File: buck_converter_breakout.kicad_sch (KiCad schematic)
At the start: 36 parts, among them J1 XT-60, J2 Conn_01x02, Q1 NMOS, Q2 PMOS, U1 MIC24066T-E/QNA

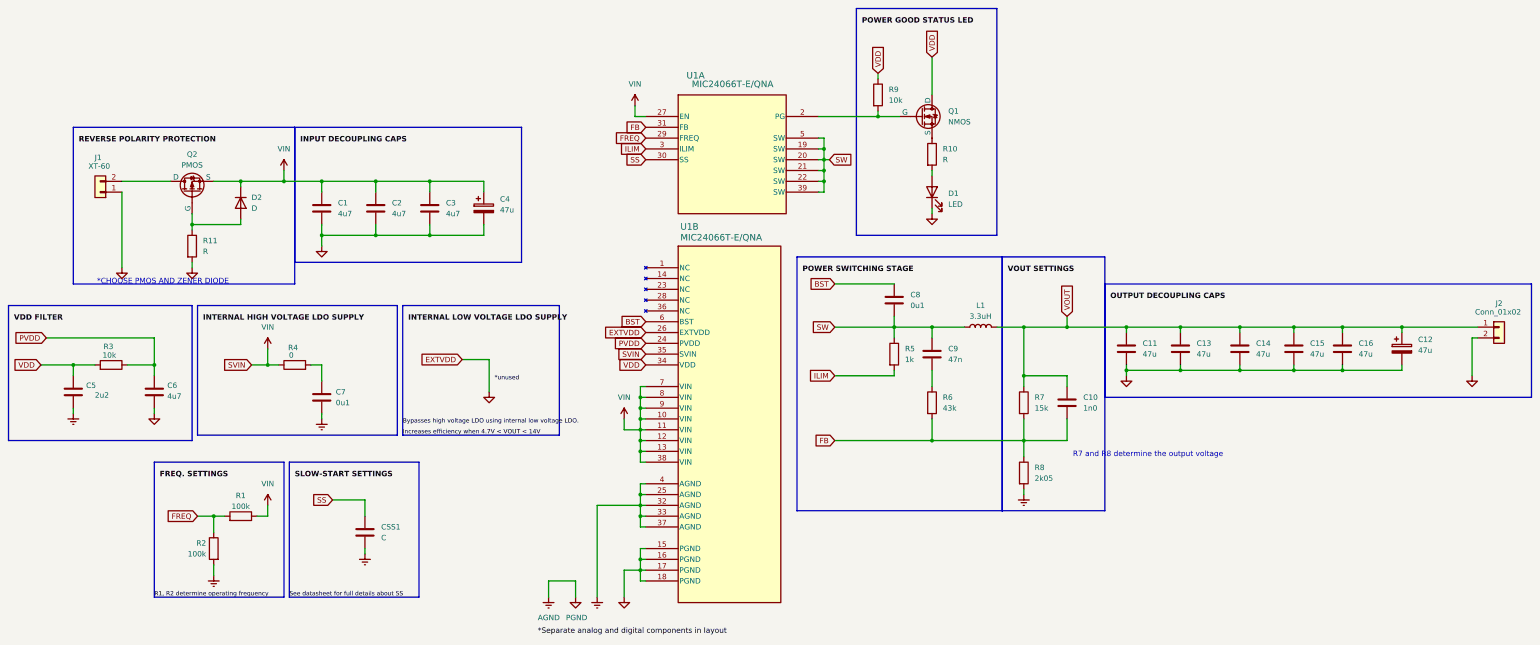
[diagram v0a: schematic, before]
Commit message: completed basic layout
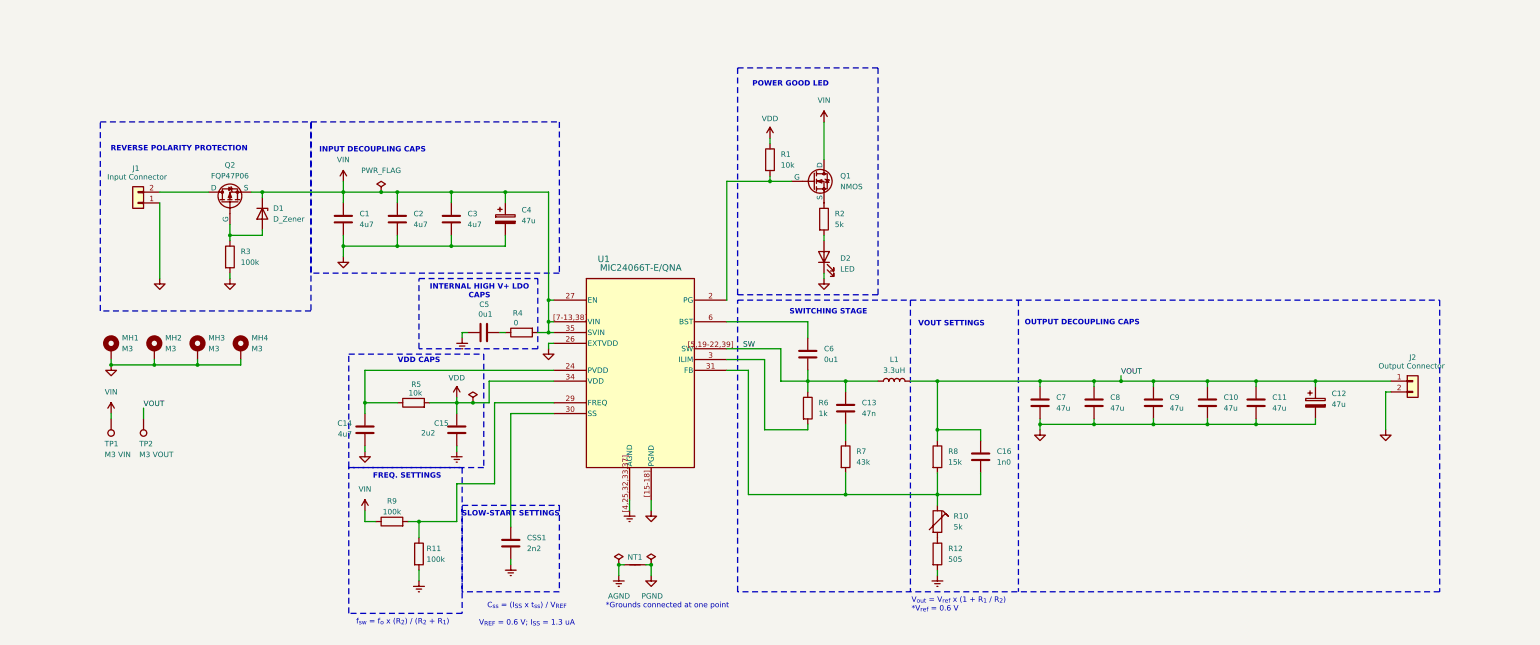
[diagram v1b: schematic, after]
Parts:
- removed D2: D, symbol Device:D
- removed unit 2 of U1
- added D1: D_Zener, Diode_SMD:D_SOD-323, symbol Device:D_Zener
- added MH1, MH2, MH3, MH4: M3, MountingHole:MountingHole_3.2mm_M3_ISO7380_Pad, symbol Mechanical:MountingHole_Pad
- added NT1: NetTie_2, NetTie:NetTie-2_SMD_Pad0.5mm, symbol Device:NetTie_2
- added R10: 5k, Potentiometer_SMD:Potentiometer_Bourns_3314J_Vertical, symbol Device:R_Trim
- added TP1: M3 VIN, TestPoint:TestPoint_Loop_D2.50mm_Drill1.0mm, symbol Connector:TestPoint
- added TP2: M3 VOUT, TestPoint:TestPoint_Loop_D2.50mm_Drill1.0mm, symbol Connector:TestPoint
- C1, C2, C3: footprint (none) -> Capacitor_SMD:C_1210_3225Metric
- C10: renamed from C15; footprint (none) -> Capacitor_SMD:C_1210_3225Metric
- C11: renamed from C16; footprint (none) -> Capacitor_SMD:C_1210_3225Metric
- C12, C4: footprint (none) -> Capacitor_SMD:CP_Elec_6.3x7.7
- C13: renamed from C9; footprint (none) -> Capacitor_SMD:C_0402_1005Metric
- C14: renamed from C6; footprint (none) -> Capacitor_SMD:C_01005_0402Metric
- C15: renamed from C5; footprint (none) -> Capacitor_SMD:C_0201_0603Metric
- C16: renamed from C10; footprint (none) -> Capacitor_SMD:C_0603_1608Metric
- C5: renamed from C7; footprint (none) -> Capacitor_SMD:C_0201_0603Metric
- C6: renamed from C8; footprint (none) -> Capacitor_SMD:C_0402_1005Metric
- C7: renamed from C11; footprint (none) -> Capacitor_SMD:C_1210_3225Metric
- C8: renamed from C13; footprint (none) -> Capacitor_SMD:C_1210_3225Metric
- C9: renamed from C14; footprint (none) -> Capacitor_SMD:C_1210_3225Metric
- CSS1: value C -> 2n2; footprint (none) -> Capacitor_SMD:C_0402_1005Metric
- D2: renamed from D1; footprint (none) -> Capacitor_SMD:C_0805_2012Metric
- J1: value XT-60 -> Input Connector; footprint (none) -> Connector_AMASS:AMASS_XT60-F_1x02_P7.20mm_Vertical
- J2: value Conn_01x02 -> Output Connector; footprint (none) -> Connector_AMASS:AMASS_XT60-F_1x02_P7.20mm_Vertical
- L1: footprint (none) -> Inductor_SMD:XGL6060-332MEC
- Q1: footprint (none) -> Package_TO_SOT_SMD:SOT-23-3
- Q2: value PMOS -> FQP47P06; footprint (none) -> Package_TO_SOT_THT:TO-220-3_Horizontal_TabDown
- R1: renamed from R9; footprint (none) -> Resistor_SMD:R_0603_1608Metric
- R11: renamed from R2; footprint (none) -> Resistor_SMD:R_0603_1608Metric
- R12: renamed from R8; value 2k05 -> 505; footprint (none) -> Resistor_SMD:R_0603_1608Metric
- R2: renamed from R10; value R -> 5k; footprint (none) -> Resistor_SMD:R_0603_1608Metric
- R3: renamed from R11; value R -> 100k; footprint (none) -> Resistor_SMD:R_0603_1608Metric
- R4: footprint (none) -> Resistor_SMD:R_0603_1608Metric
- R5: renamed from R3; footprint (none) -> Resistor_SMD:R_0603_1608Metric
- R6: renamed from R5; footprint (none) -> Resistor_SMD:R_0603_1608Metric
- R7: renamed from R6; footprint (none) -> Resistor_SMD:R_0603_1608Metric
- R8: renamed from R7; footprint (none) -> Resistor_SMD:R_0603_1608Metric
- R9: renamed from R1; footprint (none) -> Resistor_SMD:R_0603_1608Metric
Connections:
- net AGND: now also C5.1, U1.[4,25,32,33,37] (AGND), NT1.1; no longer C1.2, C10.2, C11.2, C12.2, C14.2, C2.2, C3.2, C4.2, C5.2, C7.2, C8.2, C9.2, D2.1 (K), J1.1 (Pin_1), J2.2 (Pin_2), R3.2
- net SW: now also U1.[5,19-22,39] (SW); no longer U1.19 (SW), U1.20 (SW), U1.21 (SW), U1.22 (SW), U1.39 (SW), U1.5 (SW)
- net VDD: now also U1.34 (VDD); no longer Q1.1 (D)
- net VIN: now also Q1.1 (D), R4.2, U1.35 (SVIN), U1.[7-13,38] (VIN), D1.1 (K), TP1.1; no longer R4.1
- net VOUT: now also TP2.1
- net at Q2.2 (G), R3.1: now also D1.2 (A)
- net BST: no longer names the net of C6.1
- net BST: now also U1.6 (BST)
- net FB: no longer names the net of C16.2, R7.2, R8.2, U1.31 (FB)
- net FB: now also R10.1; no longer R12.1
- net FREQ: no longer names the net of R11.1, R9.2, U1.29 (FREQ)
- net ILIM: no longer names the net of R6.2, U1.3 (ILIM)
- net PVDD: no longer names the net of C14.1, R5.1
- net PVDD: now also U1.24 (PVDD)
- net SS: no longer names the net of CSS1.1, U1.30 (SS)
- new net: C5.2, R4.1
- new net: R10.2, R12.1
- new net: U1.1 (NC), U1.14 (NC), U1.23 (NC), U1.28 (NC), U1.36 (NC)
- new net PGND: C1.2, C10.2, C11.2, C12.2, C14.2, C2.2, C3.2, C4.2, C7.2, C8.2, C9.2, D2.1 (K), J1.1 (Pin_1), J2.2 (Pin_2), MH1.1, MH2.1, MH3.1, MH4.1, NT1.2, R3.2, U1.26 (EXTVDD), U1.[15-18] (PGND)
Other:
- note added: "*Grounds connected at one point"
- note added: "C_{ss} = (I_{SS} x t_{ss}) / V_{REF} V_{REF} = 0.6 V; I_{SS} = 1.3 uA"
- note added: "FREQ. SETTINGS"
- note added: "INPUT DECOUPLING CAPS"
- note added: "INTERNAL HIGH V+ LDO CAPS"
- note added: "OUTPUT DECOUPLING CAPS"
- note added: "POWER GOOD LED"
- note added: "REVERSE POLARITY PROTECTION"
- note added: "SLOW-START SETTINGS"
- note added: "SWITCHING STAGE"
- note added: "VDD CAPS"
- note added: "VOUT SETTINGS"
- note added: "V_{out} = V_{ref} x (1 + R_{1} / R_{2}) *V_{ref} = 0.6 V"
- note added: "f_{sw} = f_{o} x (R_{2}) / (R_{2} + R_{1})"
- note removed: "*CHOOSE PMOS AND ZENER DIODE"
- note removed: "R7 and R8 determine the output voltage"
- company: (none) -> Scott Chen
- moved on the sheet: C1, C10, C11, C12, C13, C14, C15, C16, C2, C3, C4, C5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
